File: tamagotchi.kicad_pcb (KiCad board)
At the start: 2 copper layers, 34 x 34 mm, 63 parts, among them J1 Conn_01x04_Socket, J2 USB_C_Receptacle_USB2.0_16P, J3 PAD x4, Q1 AO3401A, Q2 2N7002, SW1 SW_SPDT, U1 TP4057-42-SOT26-R, U2 STM32F103C8T6, U3 XC6206P332MR-G, U4 H5VU10BB, U5 H5VU10BB, Y1 16Mhz

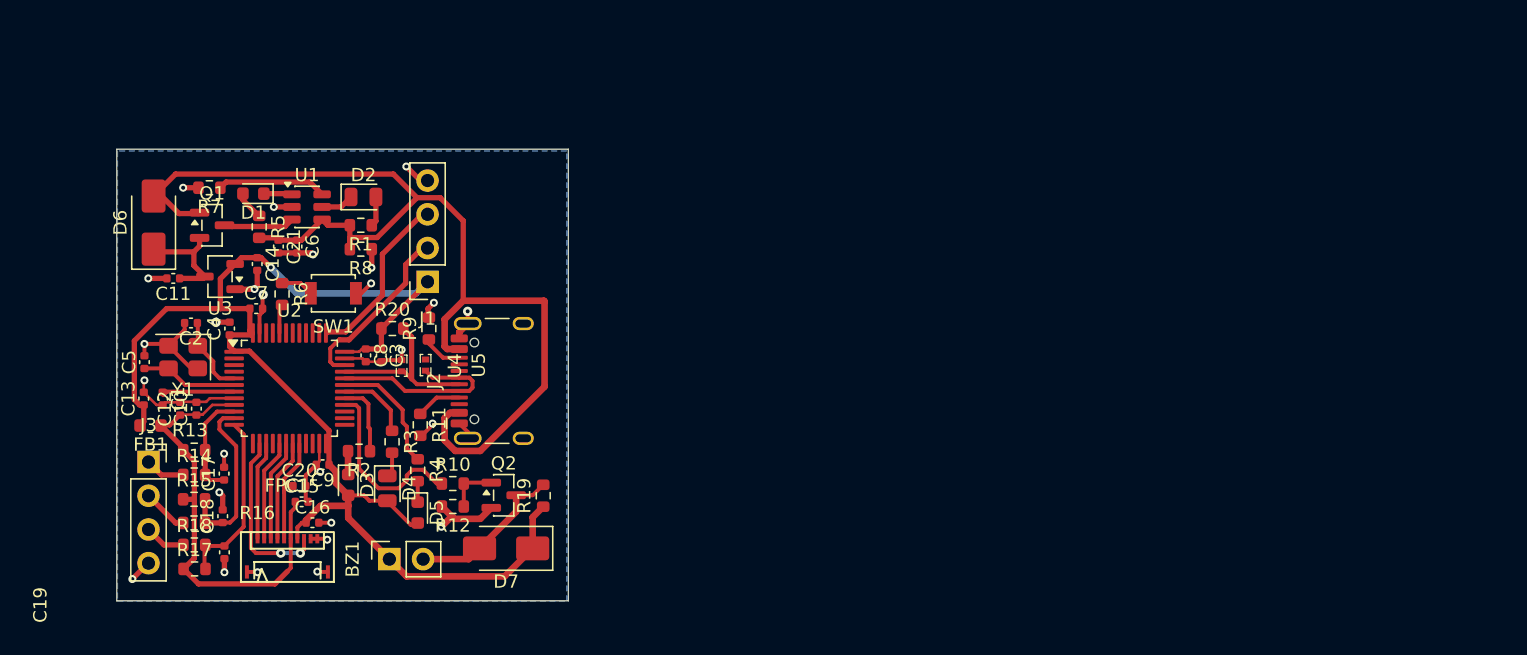
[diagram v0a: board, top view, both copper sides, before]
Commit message: fin
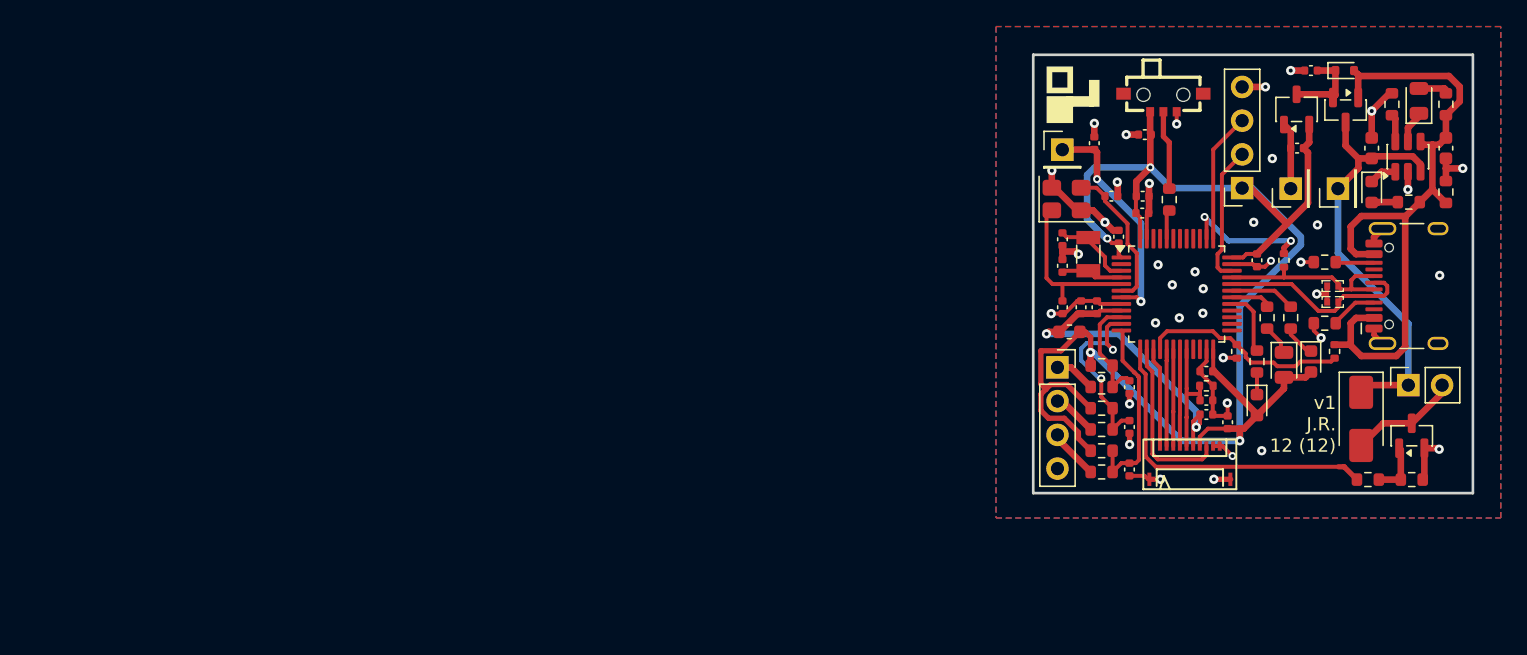
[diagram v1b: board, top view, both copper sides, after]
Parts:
- added C22: 10u, Capacitor_SMD:C_0603_1608Metric, F.Cu at (173.5, 46.4)
- added C23: 1u, Capacitor_SMD:C_0402_1005Metric, F.Cu at (168.9, 40.6)
- added J4: Conn_01x04_Socket, Connector_PinSocket_2.54mm:PinSocket_1x04_P2.54mm_Vertical, F.Cu at (163.7, 49.4)
- added J5: BAT-, Connector_PinHeader_2.54mm:PinHeader_1x01_P2.54mm_Vertical, F.Cu at (167.4, 49.5)
- added J6: BAT+, Connector_PinHeader_2.54mm:PinHeader_1x01_P2.54mm_Vertical, F.Cu at (170.9, 49.5)
- added R21: 5.1k, Resistor_SMD:R_0603_1608Metric, F.Cu at (179.1, 49.7)
- added R22: 6.8k, Resistor_SMD:R_0603_1608Metric, F.Cu at (175.0, 43.1)
- added Y2: 32.768kHz, Crystal:Crystal_SMD_3215-2Pin_3.2x1.5mm, F.Cu at (152.1, 54.4)
- C1: value 100n -> 4.7u
- C10: value 10n -> 1u
- C11, C12, C15: value 1u -> 100n
- C13, C14: value 1u -> 10p
- C16: value 1u -> 5.6p
- C17: value 100n -> 5.6p
- C2, C5: value 10p -> 100n
- C20: value 100n -> 10u; footprint Capacitor_SMD:C_0402_1005Metric -> Capacitor_SMD:C_0603_1608Metric
- C21: value 10u -> 1u
- C3: value 4.7u -> 100n
- C6: value 2.2u -> 10n
- C7, C8, C9: value 100n -> 1u
- D3: value KT-0603R -> KT-0603W
- D4: value KT-0805G -> SS14; footprint LED_SMD:LED_0805_2012Metric -> Diode_SMD:D_SMA
- D5: value KT-0603W -> RB520S-30; footprint LED_SMD:LED_0603_1608Metric -> Diode_SMD:D_SOD-523
- D6: value SS14 -> KT-0805G; footprint Diode_SMD:D_SMA -> LED_SMD:LED_0805_2012Metric
- D7: value SS14 -> KT-0603R; footprint Diode_SMD:D_SMA -> LED_SMD:LED_0603_1608Metric
- J1: value Conn_01x04_Socket -> NRST; footprint Connector_PinSocket_2.54mm:PinSocket_1x04_P2.54mm_Vertical -> Connector_PinHeader_2.54mm:PinHeader_1x01_P2.54mm_Vertical
- Q1: value AO3401A -> AO3400A
- Q2: value 2N7002 -> AO3401A
- R1: value 1k -> 5.1k
- R10, R18, R4: value 100 -> 5.1k
- R11, R13, R17: value 5.1k -> 100
- R12: value 5.1k -> 150
- R2: value 130 -> 100k; footprint Resistor_SMD:R_0603_1608Metric -> Resistor_SMD:R_0402_1005Metric
- R20: value 5.1k -> 1k
- R3: value 100 -> 100k; footprint Resistor_SMD:R_0603_1608Metric -> Resistor_SMD:R_0402_1005Metric
- R5: value 1k -> 100
- R6: value 5.1k -> 1.5k; footprint Resistor_SMD:R_0603_1608Metric -> Resistor_SMD:R_0402_1005Metric
- R7: value 2k -> 5.1k
- R9: value 5.1k -> 100k; footprint Resistor_SMD:R_0603_1608Metric -> Resistor_SMD:R_0402_1005Metric
- SW1: value SW_SPDT -> SSAJ110100; footprint Button_Switch_SMD:SW_SPST_B3U-1000P -> easyECADDownloader:SW-SMD_SSAJ110100
- U1: value TP4057-42-SOT26-R -> STM32F103C8T6; footprint Package_TO_SOT_SMD:TSOT-23-6 -> Package_QFP:LQFP-48_7x7mm_P0.5mm
- U2: value STM32F103C8T6 -> H5VU10BB; footprint Package_QFP:LQFP-48_7x7mm_P0.5mm -> easyECADDownloader:DFN1006-2L-BI
- U3: value XC6206P332MR-G -> H5VU10BB; footprint Package_TO_SOT_SMD:SOT-23-3 -> easyECADDownloader:DFN1006-2L-BI
- U4: value H5VU10BB -> XC6206P332MR-G; footprint easyECADDownloader:DFN1006-2L-BI -> Package_TO_SOT_SMD:SOT-23-3
- U5: value H5VU10BB -> TP4057-42-SOT26-R; footprint easyECADDownloader:DFN1006-2L-BI -> Package_TO_SOT_SMD:TSOT-23-6
- moved D6 95.7 mm to (177.0, 42.9)
- moved R18 91.8 mm to (176.5, 71.4)
- moved Q1 91.7 mm to (176.5, 68.1), turned to 90 degrees
- moved C20 90.0 mm to (179.1, 46.4), turned to -90 degrees
- moved R17 88.6 mm to (173.2, 71.4)
- moved R7 84.2 mm to (169.9, 55.0)
- moved U3 83.8 mm to (170.5, 58.0), turned to 0 degrees
- moved R14 83.4 mm to (167.4, 59.2), turned to -90 degrees
- moved R13 81.4 mm to (165.6, 59.2), turned to -90 degrees
- moved U2 78.9 mm to (170.5, 56.8)
- moved C11 78.3 mm to (161.0, 65.4), turned to 0 degrees
- moved BZ1 77.8 mm to (176.2, 64.3)
- moved C10 77.6 mm to (162.6, 67.1)
- moved D5 77.3 mm to (171.4, 40.6), turned to 0 degrees
- moved D1 77.2 mm to (164.8, 65.8), turned to -90 degrees
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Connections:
- BZ1 pad 1: VDD -> +BATT
- C1 pad 1: /NRST -> VDD
- C10 pad 1: VDDA -> VDD
- C11 pad 1: /REG_LDO -> /DISP_DISP
- C12 pad 1: VDDA -> /NRST
- C13 pad 1: VDD -> /HSE_IN
- C14 pad 1: VDD -> /HSE_OUT
- C15 pad 1: VDDA -> /BUT1
- C16 pad 1: VDD -> Net-(U1-PC14)
- C17 pad 1: /BUT1 -> Net-(U1-PC15)
- C2 pad 1: /HSE_IN -> VDD
- C20 pad 1: /DISP_DISP -> +5V
- C21 pad 1: +5V -> VDD
- C5 pad 1: /HSE_OUT -> VDD
- C6 pad 1: +5V -> VDDA
- C7 pad 1: VDD -> VDDA
- C9 pad 1: VDD -> VDDA
- D1 pad 1: /REG_CHRG -> Net-(D1-K)
- D1 pad 2: Net-(D1-A) -> VDD
- D2 pad 1: /REG_STBY -> Net-(D2-K)
- D2 pad 2: Net-(D2-A) -> VDD
- D4 pad 1: Net-(D4-K) -> +BATT
- D4 pad 2: VDD -> /BUZ_DRAIN
- D5 pad 2: VDD -> +5V
- D6 pad 1: /REG_LDO -> /REG_STBY
- D6 pad 2: +5V -> Net-(D6-A)
- D7 pad 1: VDD -> /REG_CHRG
- D7 pad 2: /BUZ_DRAIN -> Net-(D7-A)
- J1 pad 1: VDD -> /NRST
- Q1 pad 1: +5V -> /BUZ_GATE
- Q1 pad 2: /REG_LDO -> GND
- Q1 pad 3: +BATT -> /BUZ_DRAIN
- Q2 pad 1: /BUZ_GATE -> +5V
- Q2 pad 2: GND -> Net-(D5-K)
- Q2 pad 3: /BUZ_DRAIN -> +BATT
- R1 pad 1: Net-(D2-A) -> /BOOT0_SW
- R1 pad 2: +5V -> /BOOT0
- R10 pad 1: /BUZ -> VDD
- R10 pad 2: /BUZ_GATE -> /BUT2
- R11 pad 1: /USB_CC1 -> /BUT2_SW
- R11 pad 2: GND -> /BUT2
- R12 pad 1: /BUZ_GATE -> /LED_R
- R12 pad 2: GND -> Net-(D1-K)
- R13 pad 1: VDDA -> /LED_G
- R13 pad 2: /BUT1 -> Net-(D2-K)
- R14 pad 1: /BUT1_SW -> /LED_B
- R14 pad 2: /BUT1 -> Net-(D3-K)
- R15 pad 1: VDDA -> VDD
- R15 pad 2: /BUT2 -> /BUT3
- R16 pad 1: /BUT2_SW -> /BUT3_SW
- R16 pad 2: /BUT2 -> /BUT3
- R17 pad 1: VDDA -> /BUZ
- R17 pad 2: /BUT3 -> /BUZ_GATE
- R18 pad 1: /BUT3_SW -> /BUZ_GATE
- R18 pad 2: /BUT3 -> GND
- R19 pad 1: VDD -> Net-(D6-A)
- R19 pad 2: /BUZ_DRAIN -> +5V
- R2 pad 1: /LED_R -> Net-(U1-PA6)
- R2 pad 2: Net-(D3-K) -> +5V
- R20 pad 1: VDD -> Net-(D7-A)
- R20 pad 2: /USB_D+ -> +5V
- R3 pad 1: /LED_G -> Net-(U1-PA6)
- R3 pad 2: Net-(D4-K) -> GND
- R4 pad 1: /LED_B -> VDD
- R4 pad 2: Net-(D5-K) -> /BUT1
- R5 pad 1: Net-(D1-A) -> /BUT1_SW
- R5 pad 2: +5V -> /BUT1
- R6 pad 1: /BOOT0_SW -> Net-(U1-PA15)
- R6 pad 2: /BOOT0 -> /USB_D+
- R7 pad 1: /REG_PROG -> /USB_CC2
- R8 pad 1: GND -> /USB_CC1
- R8 pad 2: +5V -> GND
- R9 pad 1: /USB_CC2 -> /DISP_DISP
- U1 pad 1: /REG_CHRG -> VDD
- U1 pad 2: GND -> unconnected-(U1-PC13-Pad2)
- U1 pad 3: +BATT -> Net-(U1-PC14)
- U1 pad 4: +5V -> Net-(U1-PC15)
- U1 pad 5: /REG_STBY -> /HSE_IN
- U1 pad 6: /REG_PROG -> /HSE_OUT
- U2 pad 1: VDD -> GND
- U2 pad 2: unconnected-(U2-PC13-Pad2) -> /USB_D+
- U3 pad 2: VDD -> /USB_D-
- U4 pad 2: /USB_D+ -> VDD
- U5 pad 1: GND -> /REG_CHRG
- U5 pad 2: /USB_D- -> GND
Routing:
- net +5V: track 82.7 -> 51.6 mm
- net +BATT: track 5.33 -> 33.1 mm
- net VDD: track 99.4 -> 126.7 mm, vias 1 -> 4
- net Net-(U1-PA6): track 0.00 -> 15.7 mm
- net /NRST: track 5.46 -> 16.9 mm, vias 0 -> 2
- net /BUZ: track 13.8 -> 24.9 mm
- net Net-(U1-PA15): track 0.00 -> 10.1 mm, vias 0 -> 2
- net /REG_LDO: track 8.51 -> 0.00 mm
- net VDDA: track 33.4 -> 25.2 mm, vias 0 -> 2
- net /HSE_IN: track 5.95 -> 12.5 mm
- net /REG_PROG: track 8.22 -> 2.09 mm
- net Net-(U1-PC14): track 0.00 -> 6.12 mm
- net Net-(D5-K): track 1.58 -> 6.31 mm
- net Net-(U1-PC15): track 0.00 -> 4.69 mm
- net /LED_B: track 9.33 -> 4.92 mm
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- added copper zone on F.Cu, net GND
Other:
- board size 34 x 34 mm -> 33.1 x 33 mm
- board text added: "v1 J.R. 12 (12)"
